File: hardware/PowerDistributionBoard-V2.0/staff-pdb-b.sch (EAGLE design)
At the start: 5 parts, among them J3 B5B-XH-A(LF)(SN)

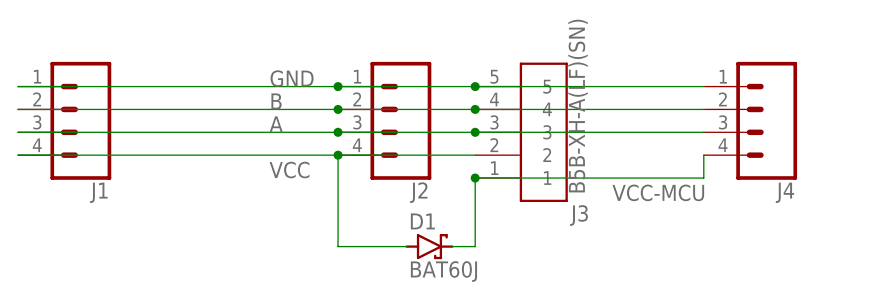
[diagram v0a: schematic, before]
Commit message: rearranging files
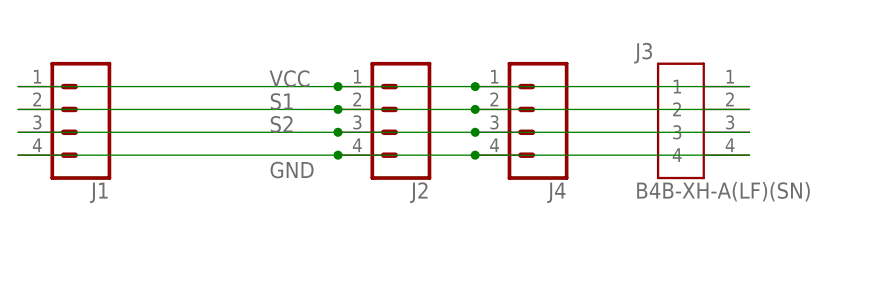
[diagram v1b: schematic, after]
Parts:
- removed D1: BAT60J, diode:BAT60J
- J3: value B5B-XH-A(LF)(SN) -> B4B-XH-A(LF)(SN); device B4B-XH-A_LF__SN_:B5B-XH-A(LF)(SN) -> RoverWing-V1.5:B4B-XH-A(LF)(SN)
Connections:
- net A renamed S2
- removed net B: J1.2, J2.2, J3.4, J4.2
- removed net VCC-MCU: D1.C, J3.1, J4.4
- new net S1: J1.2, J2.2, J3.2, J4.2
- net GND: now also J1.4, J2.4, J3.4, J4.4; no longer J1.1, J2.1, J3.5, J4.1
- net VCC: now also J1.1, J2.1, J3.1, J4.1; no longer D1.A, J1.4, J2.4, J3.2
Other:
- moved on the sheet: J4
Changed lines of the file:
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@@
 <part name="J2" library="RoverWing-cover-V1.6" deviceset="CONN_04" device=""/>
 <part name="J1" library="RoverWing-cover-V1.6" deviceset="CONN_04" device=""/>
-<part name="J3" library="B4B-XH-A_LF__SN_" deviceset="B5B-XH-A(LF)(SN)" device=""/>
+<part name="J3" library="RoverWing-V1.5" deviceset="B4B-XH-A(LF)(SN)" device=""/>
 <part name="J4" library="RoverWing-cover-V1.6" deviceset="CONN_04" device=""/>
-<part name="D1" library="diode" library_urn="urn:adsk.eagle:library:210" deviceset="BAT60J" device="" package3d_urn="urn:adsk.eagle:package:43461/1"/>
 </parts>
 <sheets>
@@
 <attribute name="NAME" x="33.02" y="75.692" size="1.778" layer="95" font="vector" rot="R180"/>
 </instance>
-<instance part="J3" gate="G$1" x="81.28" y="81.28" smashed="yes" rot="R180">
-<attribute name="VALUE" x="84.074" y="93.98" size="1.778" layer="96" font="vector" rot="R270"/>
-<attribute name="NAME" x="86.36" y="73.152" size="1.778" layer="95" font="vector" rot="R180"/>
+<instance part="J3" gate="G$1" x="96.52" y="81.28" smashed="yes">
+<attribute name="VALUE" x="91.44" y="73.914" size="1.778" layer="96" font="vector"/>
+<attribute name="NAME" x="91.44" y="89.408" size="1.778" layer="95" font="vector"/>
 </instance>
-<instance part="J4" gate="G$1" x="104.14" y="83.82" smashed="yes" rot="R180">
-<attribute name="VALUE" x="109.22" y="91.186" size="1.778" layer="96" font="vector" rot="R180"/>
-<attribute name="NAME" x="109.22" y="75.692" size="1.778" layer="95" font="vector" rot="R180"/>
-</instance>
-<instance part="D1" gate="G$1" x="68.58" y="68.58" smashed="yes">
-<attribute name="NAME" x="66.294" y="70.485" size="1.778" layer="95"/>
-<attribute name="VALUE" x="66.294" y="65.151" size="1.778" layer="96"/>
+<instance part="J4" gate="G$1" x="78.74" y="83.82" smashed="yes" rot="R180">
+<attribute name="VALUE" x="83.82" y="91.186" size="1.778" layer="96" font="vector" rot="R180"/>
+<attribute name="NAME" x="83.82" y="75.692" size="1.778" layer="95" font="vector" rot="R180"/>
 </instance>
 </instances>
@@
 </busses>
 <nets>
-<net name="GND" class="0">
+<net name="S1" class="0">
+<segment>
+<pinref part="J2" gate="G$1" pin="2"/>
+<pinref part="J1" gate="G$1" pin="2"/>
+<wire x1="22.86" y1="83.82" x2="58.42" y2="83.82" width="0.1524" layer="91"/>
+<pinref part="J4" gate="G$1" pin="2"/>
+<wire x1="58.42" y1="83.82" x2="73.66" y2="83.82" width="0.1524" layer="91"/>
+<junction x="58.42" y="83.82"/>
+<label x="50.8" y="83.82" size="1.778" layer="95"/>
+<pinref part="J3" gate="G$1" pin="2"/>
+<wire x1="73.66" y1="83.82" x2="104.14" y2="83.82" width="0.1524" layer="91"/>
+<junction x="73.66" y="83.82"/>
+</segment>
+</net>
+<net name="S2" class="0">
+<segment>
+<pinref part="J2" gate="G$1" pin="3"/>
+<pinref part="J1" gate="G$1" pin="3"/>
+<wire x1="22.86" y1="81.28" x2="58.42" y2="81.28" width="0.1524" layer="91"/>
+<pinref part="J4" gate="G$1" pin="3"/>
+<wire x1="58.42" y1="81.28" x2="73.66" y2="81.28" width="0.1524" layer="91"/>
+<junction x="58.42" y="81.28"/>
+<label x="50.8" y="81.28" size="1.778" layer="95"/>
+<pinref part="J3" gate="G$1" pin="3"/>
+<wire x1="73.66" y1="81.28" x2="104.14" y2="81.28" width="0.1524" layer="91"/>
+<junction x="73.66" y="81.28"/>
+</segment>
+</net>
+<net name="VCC" class="0">
 <segment>
 <pinref part="J2" gate="G$1" pin="1"/>
@@
 <wire x1="22.86" y1="86.36" x2="58.42" y2="86.36" width="0.1524" layer="91"/>
 <label x="50.8" y="86.36" size="1.778" layer="95"/>
-<pinref part="J3" gate="G$1" pin="5"/>
+<pinref part="J4" gate="G$1" pin="1"/>
 <wire x1="58.42" y1="86.36" x2="73.66" y2="86.36" width="0.1524" layer="91"/>
 <junction x="58.42" y="86.36"/>
-<pinref part="J4" gate="G$1" pin="1"/>
-<wire x1="73.66" y1="86.36" x2="99.06" y2="86.36" width="0.1524" layer="91"/>
+<pinref part="J3" gate="G$1" pin="1"/>
+<wire x1="73.66" y1="86.36" x2="104.14" y2="86.36" width="0.1524" layer="91"/>
 <junction x="73.66" y="86.36"/>
 </segment>
 </net>
-<net name="B" class="0">
-<segment>
-<pinref part="J2" gate="G$1" pin="2"/>
-<pinref part="J1" gate="G$1" pin="2"/>
-<wire x1="22.86" y1="83.82" x2="58.42" y2="83.82" width="0.1524" layer="91"/>
-<label x="50.8" y="83.82" size="1.778" layer="95"/>
-<pinref part="J3" gate="G$1" pin="4"/>
-<wire x1="58.42" y1="83.82" x2="73.66" y2="83.82" width="0.1524" layer="91"/>
-<junction x="58.42" y="83.82"/>
-<pinref part="J4" gate="G$1" pin="2"/>
-<wire x1="73.66" y1="83.82" x2="99.06" y2="83.82" width="0.1524" layer="91"/>
-<junction x="73.66" y="83.82"/>
-</segment>
-</net>
-<net name="A" class="0">
-<segment>
-<pinref part="J2" gate="G$1" pin="3"/>
-<pinref part="J1" gate="G$1" pin="3"/>
-<wire x1="22.86" y1="81.28" x2="58.42" y2="81.28" width="0.1524" layer="91"/>
-<label x="50.8" y="81.28" size="1.778" layer="95"/>
-<pinref part="J3" gate="G$1" pin="3"/>
-<wire x1="58.42" y1="81.28" x2="73.66" y2="81.28" width="0.1524" layer="91"/>
-<junction x="58.42" y="81.28"/>
-<pinref part="J4" gate="G$1" pin="3"/>
-<wire x1="73.66" y1="81.28" x2="99.06" y2="81.28" width="0.1524" layer="91"/>
-<junction x="73.66" y="81.28"/>
-</segment>
-</net>
-<net name="VCC" class="0">
+<net name="GND" class="0">
 <segment>
 <pinref part="J2" gate="G$1" pin="4"/>
@@
 <wire x1="22.86" y1="78.74" x2="58.42" y2="78.74" width="0.1524" layer="91"/>
 <label x="50.8" y="76.2" size="1.778" layer="95"/>
-<pinref part="J3" gate="G$1" pin="2"/>
+<pinref part="J4" gate="G$1" pin="4"/>
 <wire x1="58.42" y1="78.74" x2="73.66" y2="78.74" width="0.1524" layer="91"/>
 <junction x="58.42" y="78.74"/>
-<pinref part="D1" gate="G$1" pin="A"/>
-<wire x1="58.42" y1="78.74" x2="58.42" y2="68.58" width="0.1524" layer="91"/>
-<wire x1="58.42" y1="68.58" x2="66.04" y2="68.58" width="0.1524" layer="91"/>
-</segment>
-</net>
-<net name="VCC-MCU" class="0">
-<segment>
-<pinref part="J3" gate="G$1" pin="1"/>
-<wire x1="73.66" y1="76.2" x2="99.06" y2="76.2" width="0.1524" layer="91"/>
-<pinref part="J4" gate="G$1" pin="4"/>
-<wire x1="99.06" y1="76.2" x2="99.06" y2="78.74" width="0.1524" layer="91"/>
-<pinref part="D1" gate="G$1" pin="C"/>
-<wire x1="71.12" y1="68.58" x2="73.66" y2="68.58" width="0.1524" layer="91"/>
-<wire x1="73.66" y1="68.58" x2="73.66" y2="76.2" width="0.1524" layer="91"/>
-<junction x="73.66" y="76.2"/>
-<label x="88.9" y="73.66" size="1.778" layer="95"/>
+<pinref part="J3" gate="G$1" pin="4"/>
+<wire x1="73.66" y1="78.74" x2="104.14" y2="78.74" width="0.1524" layer="91"/>
+<junction x="73.66" y="78.74"/>
 </segment>
 </net>
@@
 </schematic>
 </drawing>
-<compatibility>
-<note version="8.2" severity="warning">
-Since Version 8.2, EAGLE supports online libraries. The ids
-of those online libraries will not be understood (or retained)
-with this version.
-</note>
-<note version="8.3" severity="warning">
-Since Version 8.3, EAGLE supports URNs for individual library
-assets (packages, symbols, and devices). The URNs of those assets
-will not be understood (or retained) with this version.
-</note>
-<note version="8.3" severity="warning">
-Since Version 8.3, EAGLE supports the association of 3D packages
-with devices in libraries, schematics, and board files. Those 3D
-packages will not be understood (or retained) with this version.
-</note>
-</compatibility>
 </eagle>
